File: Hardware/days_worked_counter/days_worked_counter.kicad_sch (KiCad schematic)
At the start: 5 parts, among them J101 OUT, J102 IN, J103 OUT, J104 IN, J105 OUT

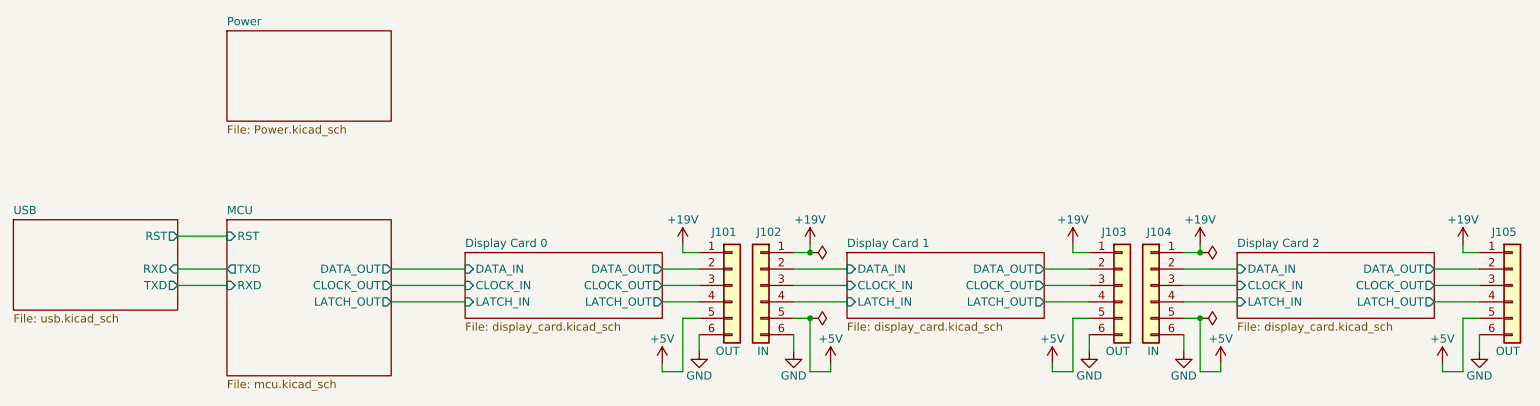
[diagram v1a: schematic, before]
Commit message: With thanks to @ka2qfx
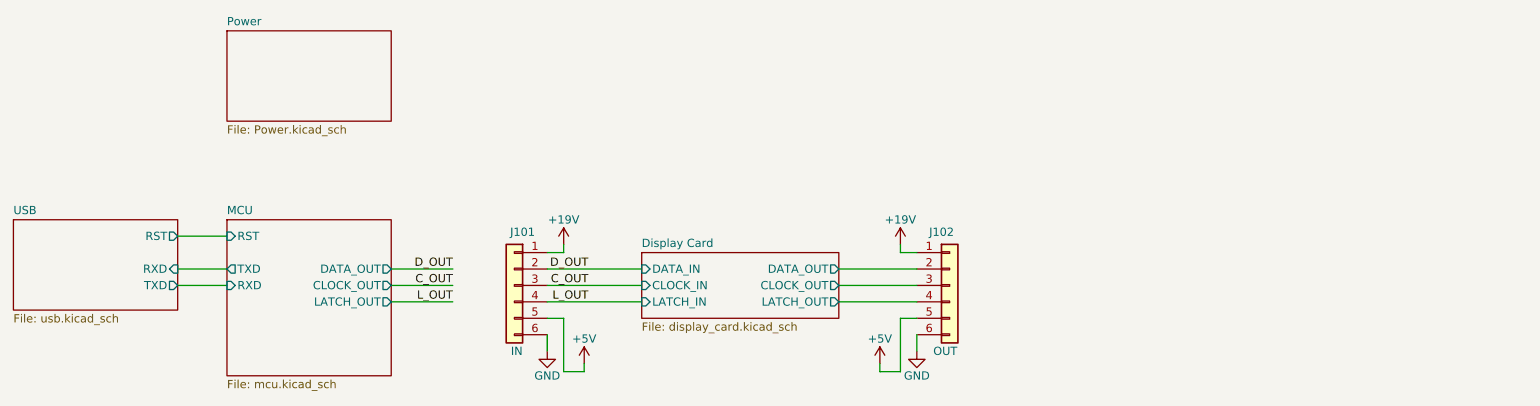
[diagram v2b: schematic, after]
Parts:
- removed J103, J105: OUT, Connector_PinSocket_2.54mm:PinSocket_1x06_P2.54mm_Vertical, symbol Connector_Generic:Conn_01x06
- removed J104: IN, Connector_PinSocket_2.54mm:PinSocket_1x06_P2.54mm_Vertical, symbol Connector_Generic:Conn_01x06
- renumbered J102 to J101, J101 to J102
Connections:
- net Display Card 1/CLOCK_IN renamed C_OUT
- net Display Card 1/DATA_IN renamed D_OUT
- net Display Card 1/LATCH_IN renamed L_OUT
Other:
- sheet Display Card 0 renamed Display Card
- removed sheet Display Card 1
- removed sheet Display Card 2
- moved on the sheet: J101, J102
